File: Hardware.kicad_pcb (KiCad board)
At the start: 2 copper layers, 133.4 x 56.1 mm, 75 parts, among them J1 Conn_02x02_Odd_Even, J10 Conn_01x04, J11 Conn_01x04, J12 Conn_02x13_Odd_Even, J2 Conn_01x04, J3 Conn_02x02_Odd_Even, J4 Conn_01x02_Male, J5 Conn_01x02_Male, J6 Conn_01x02_Male, J7 Conn_01x02_Male, J8 Conn_01x03, J9 Conn_01x03, Q1 BD140, Q10 BC548, Q11 BD139, Q12 BD139, Q2 BD140, Q3 BC548, Q4 BC548, Q5 BD139, Q6 BD139, Q7 BD140, Q8 BD140, Q9 BC548, U1 LM393, U2 TCRT5000, U3 LM324, U4 HC-05, U5 TCRT5000

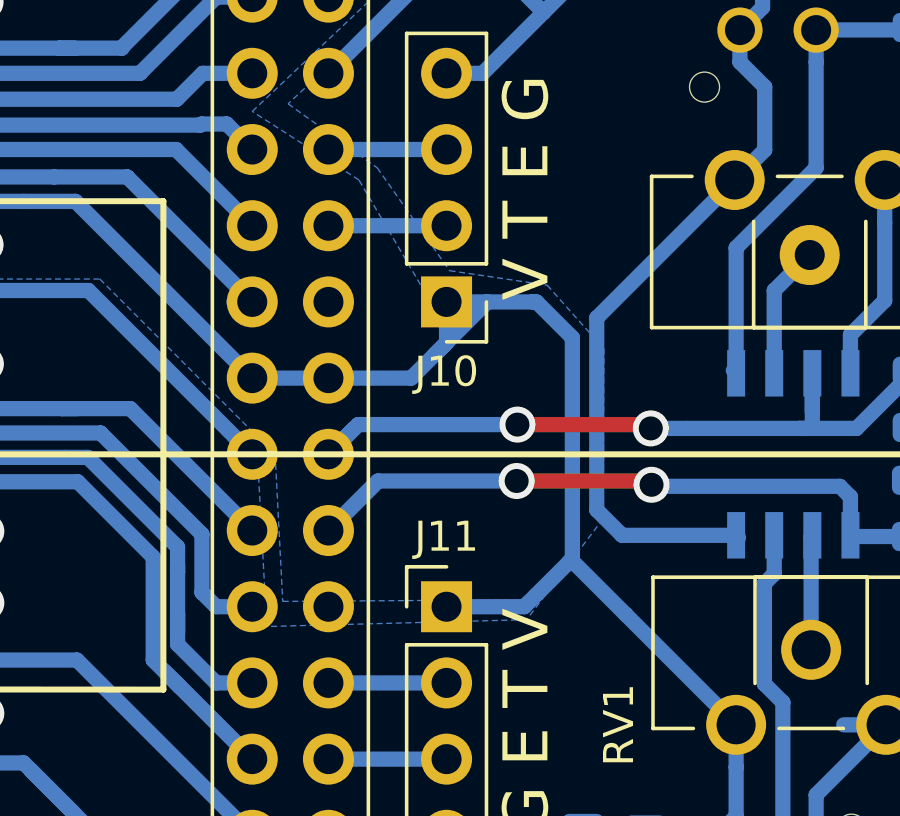
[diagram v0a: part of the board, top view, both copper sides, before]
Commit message: update
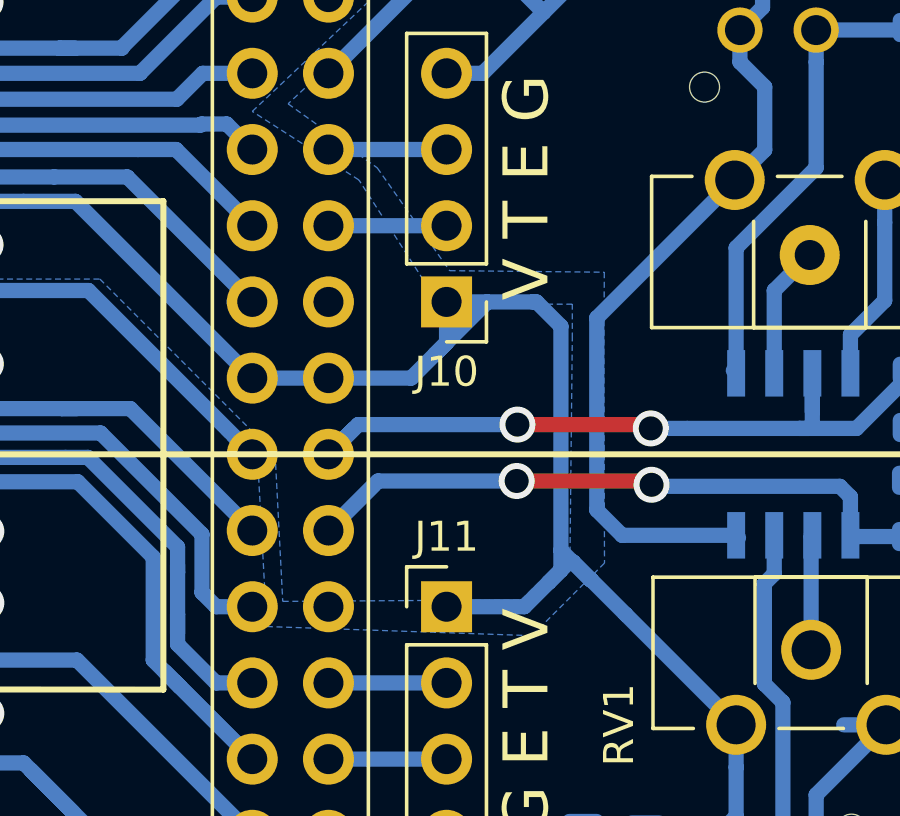
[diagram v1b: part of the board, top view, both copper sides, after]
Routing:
- net +5V: track 236.9 -> 239.0 mm
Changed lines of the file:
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@@
     (thickness 1.6)
     (drawings 48)
-    (tracks 912)
+    (tracks 917)
     (zones 0)
     (modules 75)
@@
   (via (at 165.56041 99.90141) (size 1.2) (drill 0.8) (layers F.Cu B.Cu) (net 1))
   (via (at 191.0334 95.7834) (size 1.2) (drill 0.8) (layers F.Cu B.Cu) (net 1))
-  (via (at 191.0334 101.854) (size 1.2) (drill 0.8) (layers F.Cu B.Cu) (net 1) (status 1000000))
+  (via (at 191.0334 101.854) (size 1.2) (drill 0.8) (layers F.Cu B.Cu) (net 1))
   (via (at 191.0334 98.171) (size 1.2) (drill 0.8) (layers F.Cu B.Cu) (net 1))
   (via (at 191.0184 90.2058) (size 1.2) (drill 0.8) (layers F.Cu B.Cu) (net 1))
@@
   (segment (start 212.9536 105.6894) (end 213.0044 105.7402) (width 0.508) (layer B.Cu) (net 2))
   (segment (start 210.9216 105.6894) (end 212.9536 105.6894) (width 0.508) (layer B.Cu) (net 2))
-  (segment (start 210.5683 96.6978) (end 210.4644 96.8017) (width 0.508) (layer B.Cu) (net 2))
-  (segment (start 210.5683 89.3318) (end 210.5683 96.6978) (width 0.508) (layer B.Cu) (net 2))
-  (segment (start 208.9681 98.298) (end 210.4644 96.8017) (width 0.508) (layer B.Cu) (net 2))
-  (segment (start 210.5683 89.3318) (end 209.3745 88.138) (width 0.508) (layer B.Cu) (net 2))
-  (segment (start 210.5937 96.8017) (end 212.344 98.552) (width 0.508) (layer B.Cu) (net 2))
   (segment (start 210.4644 96.8017) (end 210.5937 96.8017) (width 0.508) (layer B.Cu) (net 2))
   (segment (start 212.344 98.552) (end 216.027 102.235) (width 0.508) (layer B.Cu) (net 2))
@@
   (segment (start 213.0044 105.7402) (end 215.5698 105.7402) (width 0.508) (layer B.Cu) (net 2))
   (segment (start 215.5698 105.7402) (end 216.027 105.283) (width 0.508) (layer B.Cu) (net 2))
+  (segment (start 210.1873 97.0788) (end 209.7786 97.4875) (width 0.508) (layer B.Cu) (net 2))
+  (segment (start 209.7786 97.4875) (end 210.4644 96.8017) (width 0.508) (layer B.Cu) (net 2))
+  (segment (start 208.9681 98.298) (end 209.7786 97.4875) (width 0.508) (layer B.Cu) (net 2))
+  (segment (start 210.1873 88.9508) (end 209.3745 88.138) (width 0.508) (layer B.Cu) (net 2))
+  (segment (start 211.1779 97.409) (end 210.1873 96.4184) (width 0.508) (layer B.Cu) (net 2))
+  (segment (start 211.201 97.409) (end 211.1779 97.409) (width 0.508) (layer B.Cu) (net 2))
+  (segment (start 210.1873 96.4184) (end 210.1873 97.0788) (width 0.508) (layer B.Cu) (net 2))
+  (segment (start 210.1873 88.9508) (end 210.1873 96.4184) (width 0.508) (layer B.Cu) (net 2))
+  (segment (start 211.201 97.409) (end 212.344 98.552) (width 0.508) (layer B.Cu) (net 2))
+  (segment (start 210.5937 96.8017) (end 211.201 97.409) (width 0.508) (layer B.Cu) (net 2))
   (segment (start 199.898 88.138) (end 199.2884 88.138) (width 0.508) (layer B.Cu) (net 3))
   (segment (start 162.6489 88.309586) (end 166.986106 83.97238) (width 0.508) (layer B.Cu) (net 3))
@@
       (pts
         (xy 189.484 87.376) (xy 194.818 87.376) (xy 200.66 93.218) (xy 200.914 98.1202) (xy 208.8642 98.0694)
-        (xy 210.4898 96.4946) (xy 210.566 89.3572) (xy 209.2706 88.1888) (xy 205.994 88.392) (xy 203.454 84.074)
+        (xy 210.4898 96.4946) (xy 210.566 89.3572) (xy 210.566 88.2142) (xy 206.121 88.2142) (xy 203.454 84.074)
         (xy 199.898 81.788) (xy 204.47 77.47) (xy 204.343 73.7108) (xy 203.5556 73.0758) (xy 202.692 72.8726)
         (xy 184.404 72.644) (xy 184.404 64.516) (xy 181.356 65.024) (xy 177.038 80.01)
@@
       (pts
         (xy 185.2168 64.643) (xy 185.2168 72.1106) (xy 204.2414 72.3138) (xy 205.232 73.4314) (xy 205.3844 77.5208)
-        (xy 201.0918 81.534) (xy 204.0636 83.6676) (xy 206.4766 87.0966) (xy 209.7278 87.5792) (xy 211.6201 89.7001)
-        (xy 211.5947 95.3643) (xy 209.042 98.7298) (xy 200.3806 98.9584) (xy 200.1012 93.8022) (xy 194.4624 87.884)
+        (xy 201.0918 81.534) (xy 204.0636 83.6676) (xy 206.4766 87.0966) (xy 211.6328 87.1474) (xy 211.6201 89.7001)
+        (xy 211.63915 96.84385) (xy 209.2198 99.2632) (xy 200.3806 98.9584) (xy 200.1012 93.8022) (xy 194.4624 87.884)
         (xy 189.1792 87.9094) (xy 176.8348 80.899) (xy 176.3776 80.3656) (xy 176.7332 78.0796) (xy 165.227 78.2828)
         (xy 161.3408 83.312) (xy 156.972 84.074) (xy 155.9052 85.2424) (xy 155.8544 91.3638) (xy 158.9786 94.1832)
